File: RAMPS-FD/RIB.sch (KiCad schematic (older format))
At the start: 19 parts, among them M1 LOGO_OSHW, P1 CONN_8, P10 CONN_8, P11 CONN_8, P12 CONN_18X2, P13 CONN_10, P14 CONN_8, P15 CONN_8, P2 CONN_8, P3 CONN_8, P4 CONN_18X2, P5 CONN_10, P6 CONN_8, P7 CONN_8, P8 CONN_3X2, P9 CONN_8

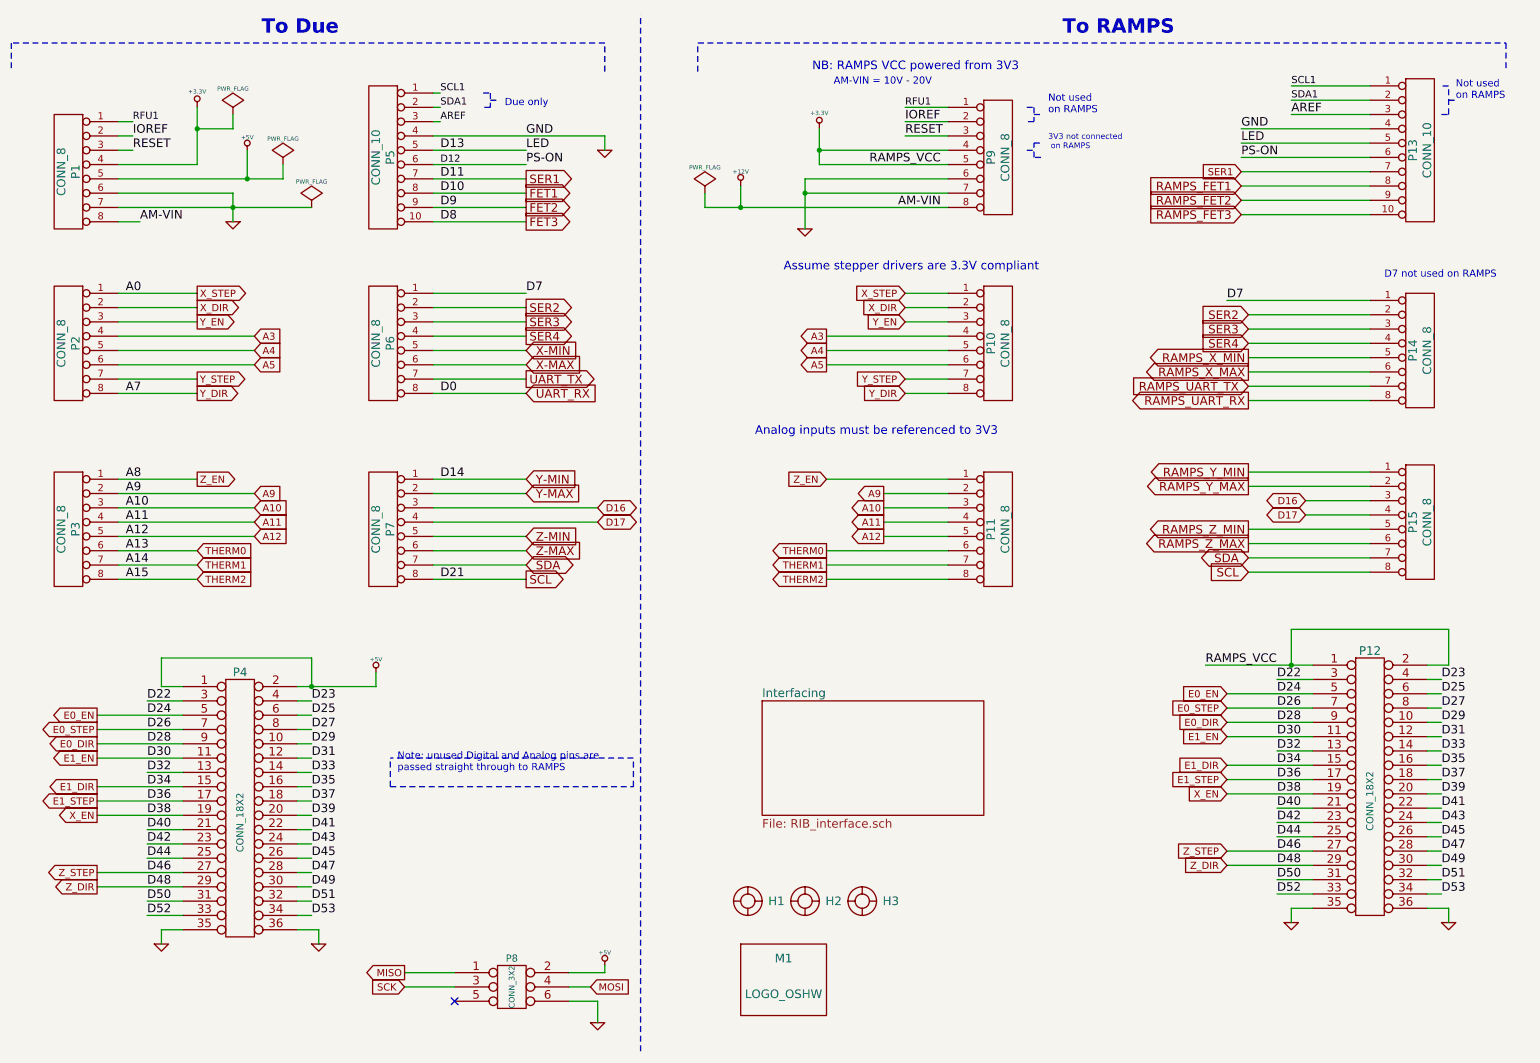
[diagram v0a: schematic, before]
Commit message: First version of RAMPS-FD, RIB
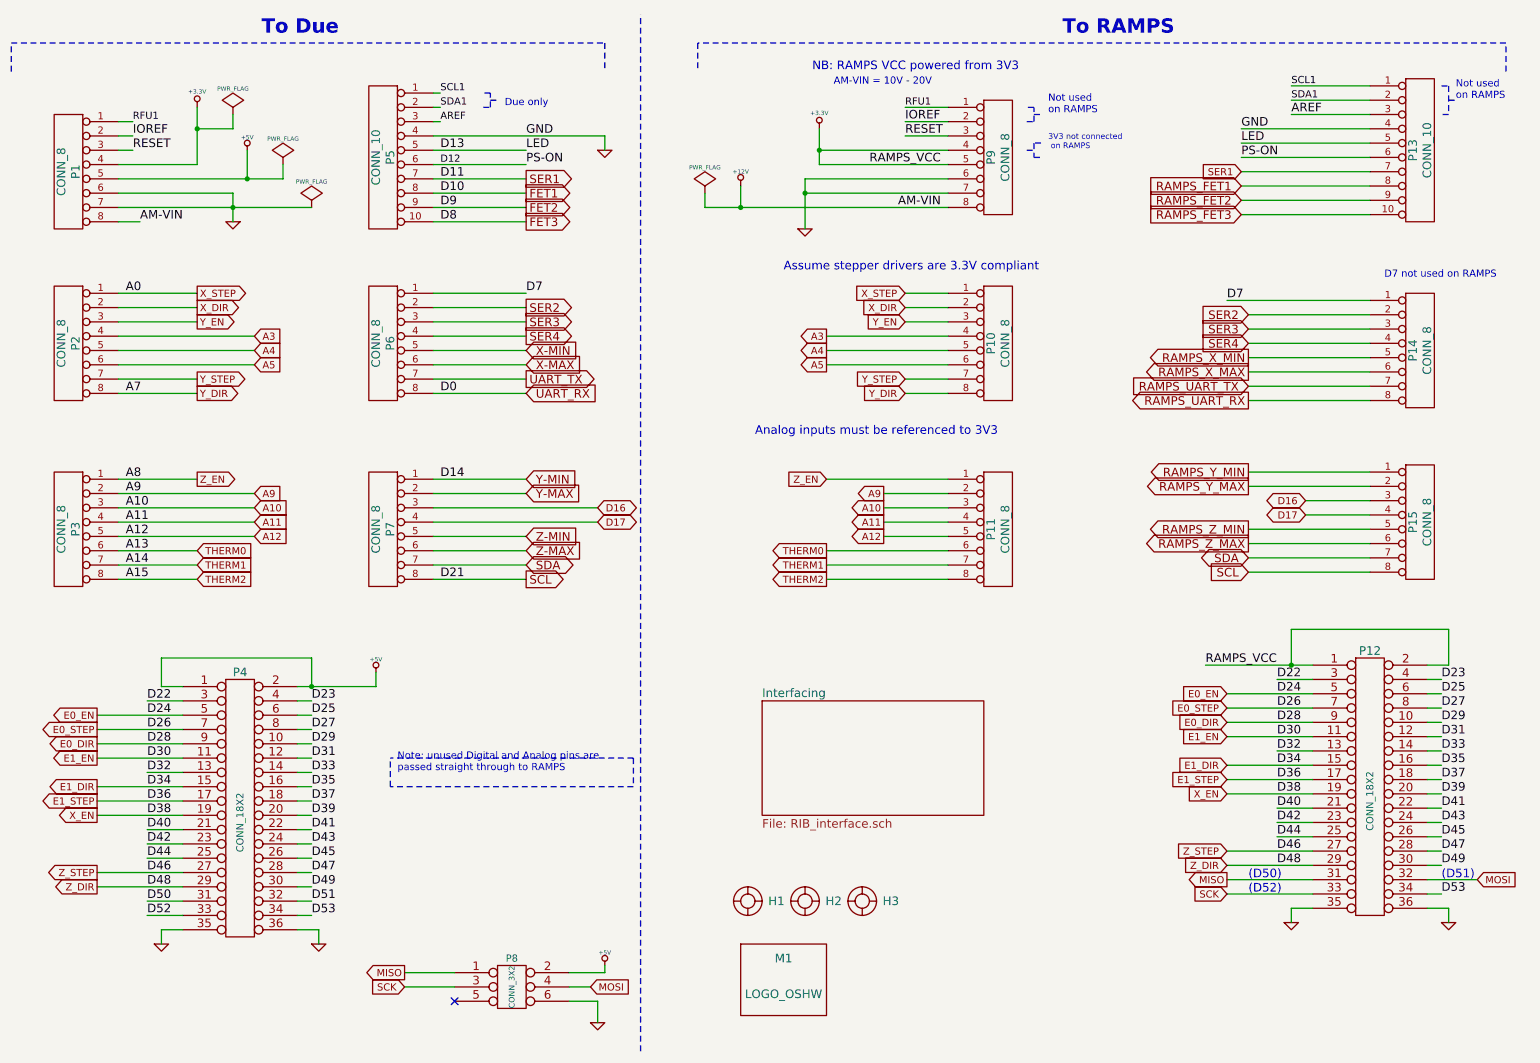
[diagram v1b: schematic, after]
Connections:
- net D50: no longer P12.31 (P31)
- net D51: no longer P12.32 (P32)
- net D52: no longer P12.33 (P33)
- net MISO: now also P12.31 (P31)
- net MOSI: now also P12.32 (P32)
- net SCK: now also P12.33 (P33)
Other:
- note added: "(D50)"
- note added: "(D51)"
- note added: "(D52)"
